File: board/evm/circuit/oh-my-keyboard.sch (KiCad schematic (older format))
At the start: 0 parts

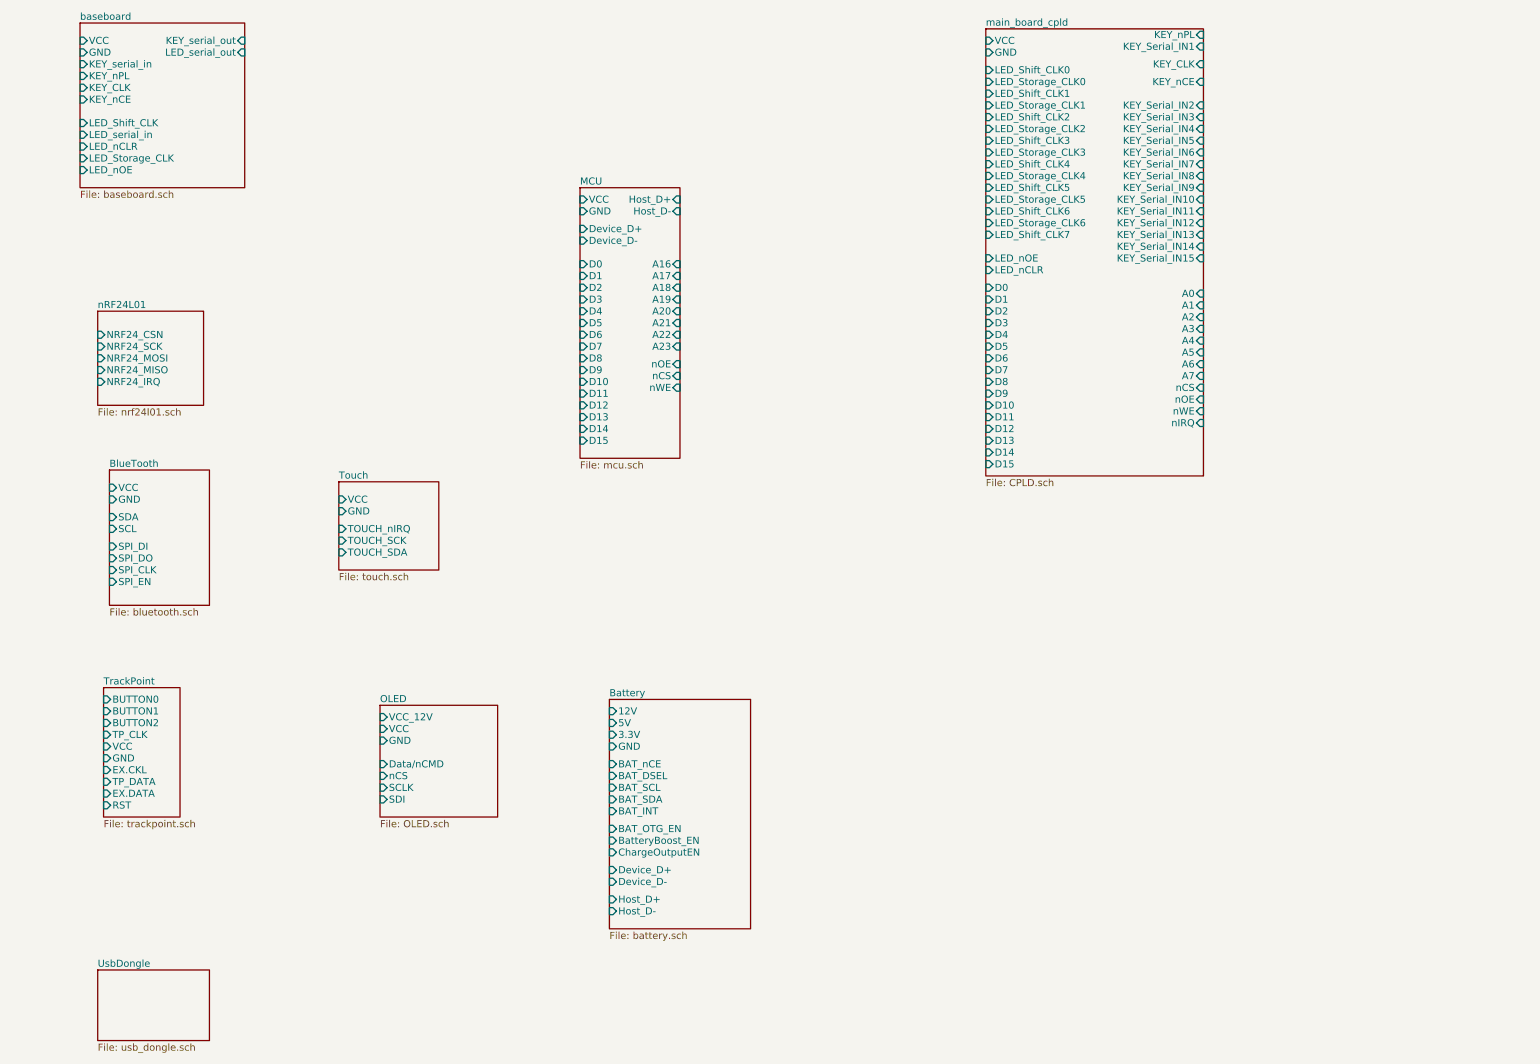
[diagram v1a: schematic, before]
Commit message: evm sch design finished
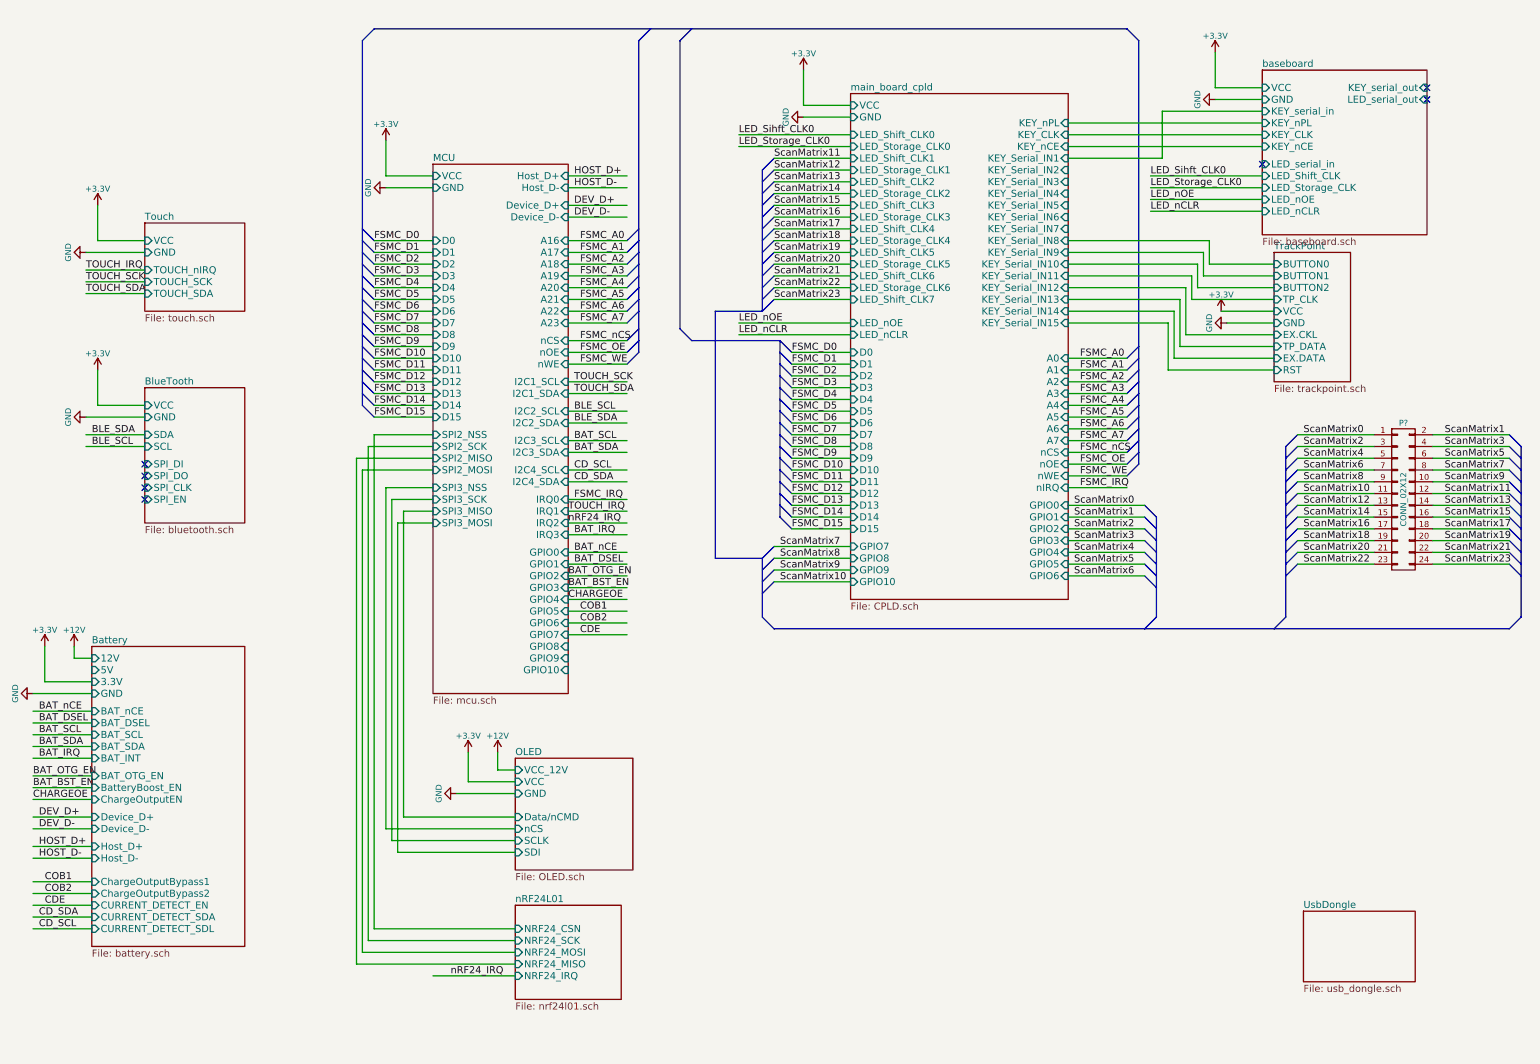
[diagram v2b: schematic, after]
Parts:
- added P?: CONN_02X12, symbol CONN_02X12
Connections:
- net labels added: +12V, +3.3V, BAT_BST_EN, BAT_DSEL, BAT_IRQ, BAT_OTG_EN, BAT_SCL, BAT_SDA, BAT_nCE, BLE_SCL, BLE_SDA, CDE, CD_SCL, CD_SDA, CHARGEOE, COB1, COB2, DEV_D+, DEV_D-, FSMC_A0, FSMC_A1, FSMC_A2, FSMC_A3, FSMC_A4, FSMC_A5, FSMC_A6, FSMC_A7, FSMC_D0, FSMC_D1, FSMC_D10, FSMC_D11, FSMC_D12, FSMC_D13, FSMC_D14, FSMC_D15, FSMC_D2, FSMC_D3, FSMC_D4, FSMC_D5, FSMC_D6, FSMC_D7, FSMC_D8, FSMC_D9, FSMC_IRQ, FSMC_OE, FSMC_WE, FSMC_nCS, GND, HOST_D+, HOST_D-, LED_Sihft_CLK0, LED_Storage_CLK0, LED_nCLR, LED_nOE, ScanMatrix0, ScanMatrix1, ScanMatrix10, ScanMatrix11, ScanMatrix12, ScanMatrix13, ScanMatrix14, ScanMatrix15, ScanMatrix16, ScanMatrix17, ScanMatrix18, ScanMatrix19, ScanMatrix2, ScanMatrix20, ScanMatrix21, ScanMatrix22, ScanMatrix23, ScanMatrix3, ScanMatrix4, ScanMatrix5, ScanMatrix6, ScanMatrix7, ScanMatrix8, ScanMatrix9, TOUCH_IRQ, TOUCH_SCK, TOUCH_SDA, nRF24_IRQ
- wire segments 0 -> 239
- no-connect marks 0 -> 7
